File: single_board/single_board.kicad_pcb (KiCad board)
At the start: 4 copper layers, 124.9 x 93.4 mm, 121 parts, among them J1 SWD, J11 SPI Debug, J17 BOOTSEL, J2 USB_C_Receptacle_USB2.0_16P, J30 JST_GH_H, J31 JST_GH_H, J32 PB_Vertical, J33 JST_GH_H, J34 PB_Vertical, J35 JST_GH_H, J36 JST_GH_H, J37 JST_GH_H, J38 PB_Vertical, J39 PB_Vertical, J4 RST, J40 PB_Vertical, J41 PB_Vertical, J42 PB_Vertical, J43 PB_Vertical, J44 PB_Vertical, J45 PB_Vertical, J46 PB_Vertical, J47 PB_Vertical, J48 PB_Vertical, J49 PB_Vertical, J5 JST-GH, J50 PB_Vertical, J6 Conn_01x02, Q1 AO3400A, Q3 AO3401A, SW1 Button, U1 AP2112K-3.3, U3 USBLC6-2SC6, U4 LSM6DSV, U5 STM32G474VBTx, Y2 ABM8-16MHz

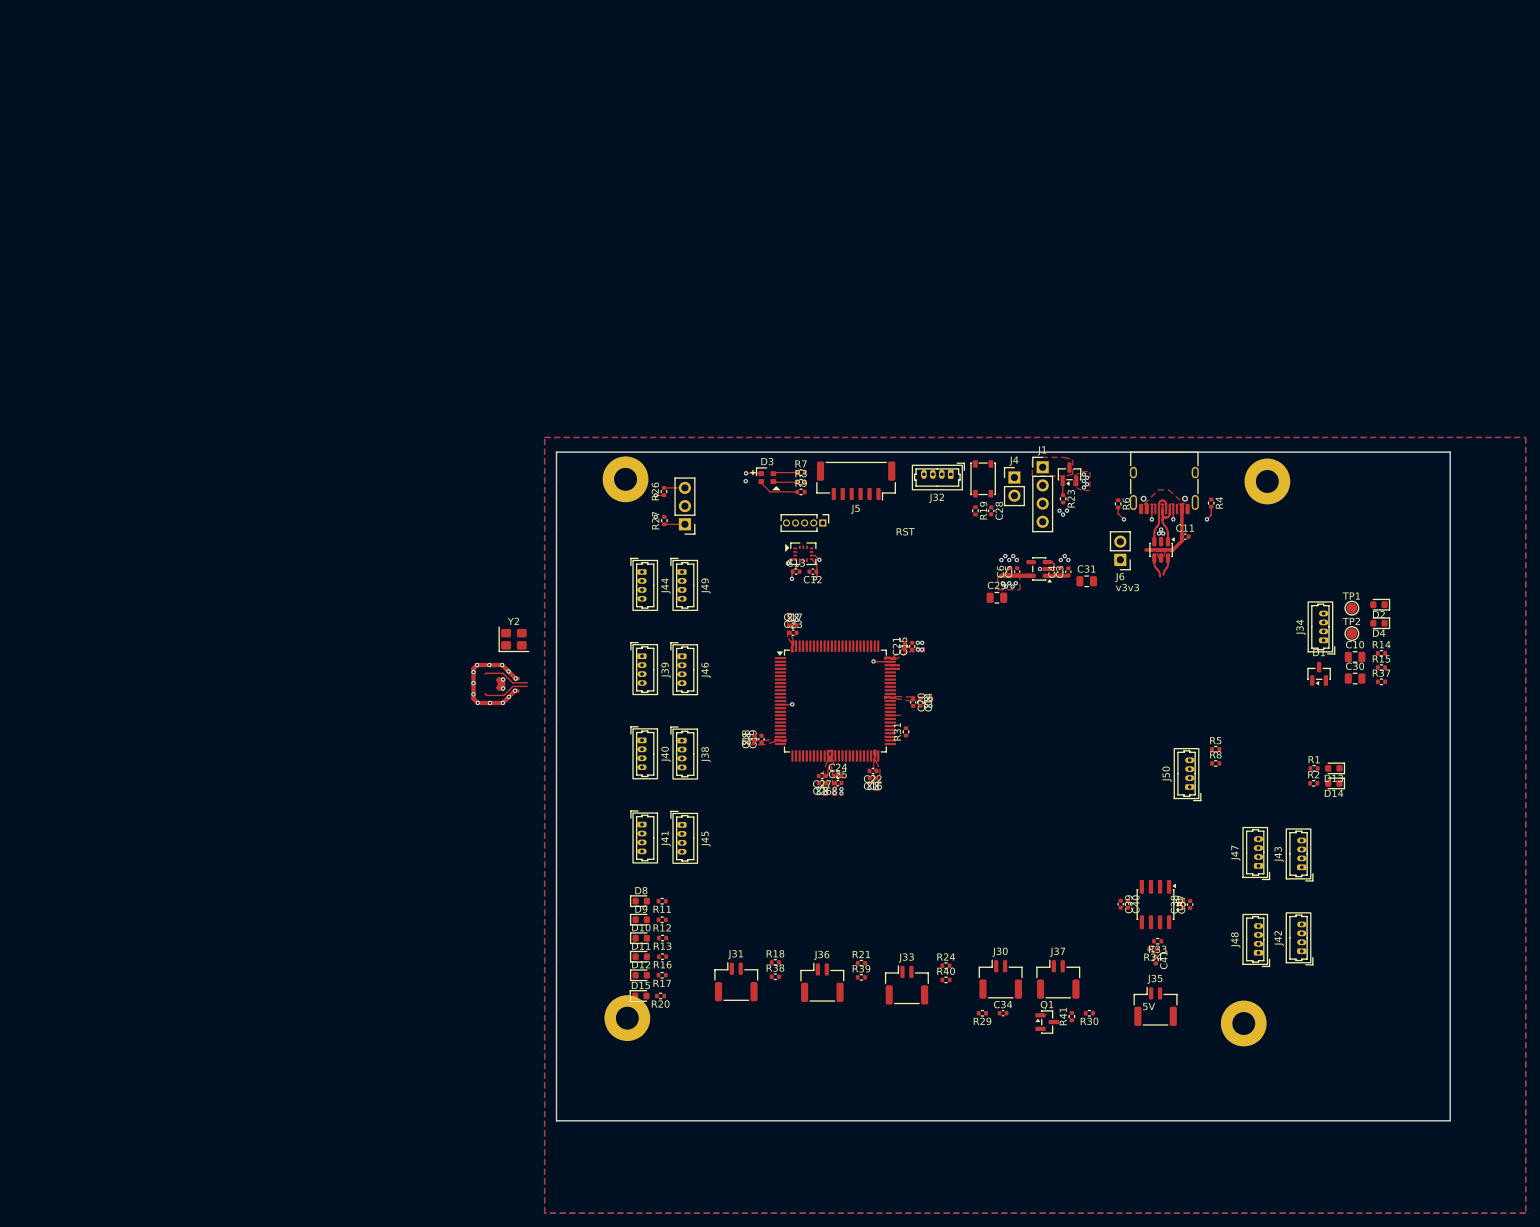
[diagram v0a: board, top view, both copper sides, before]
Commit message: layout positioning
spacing and positioning
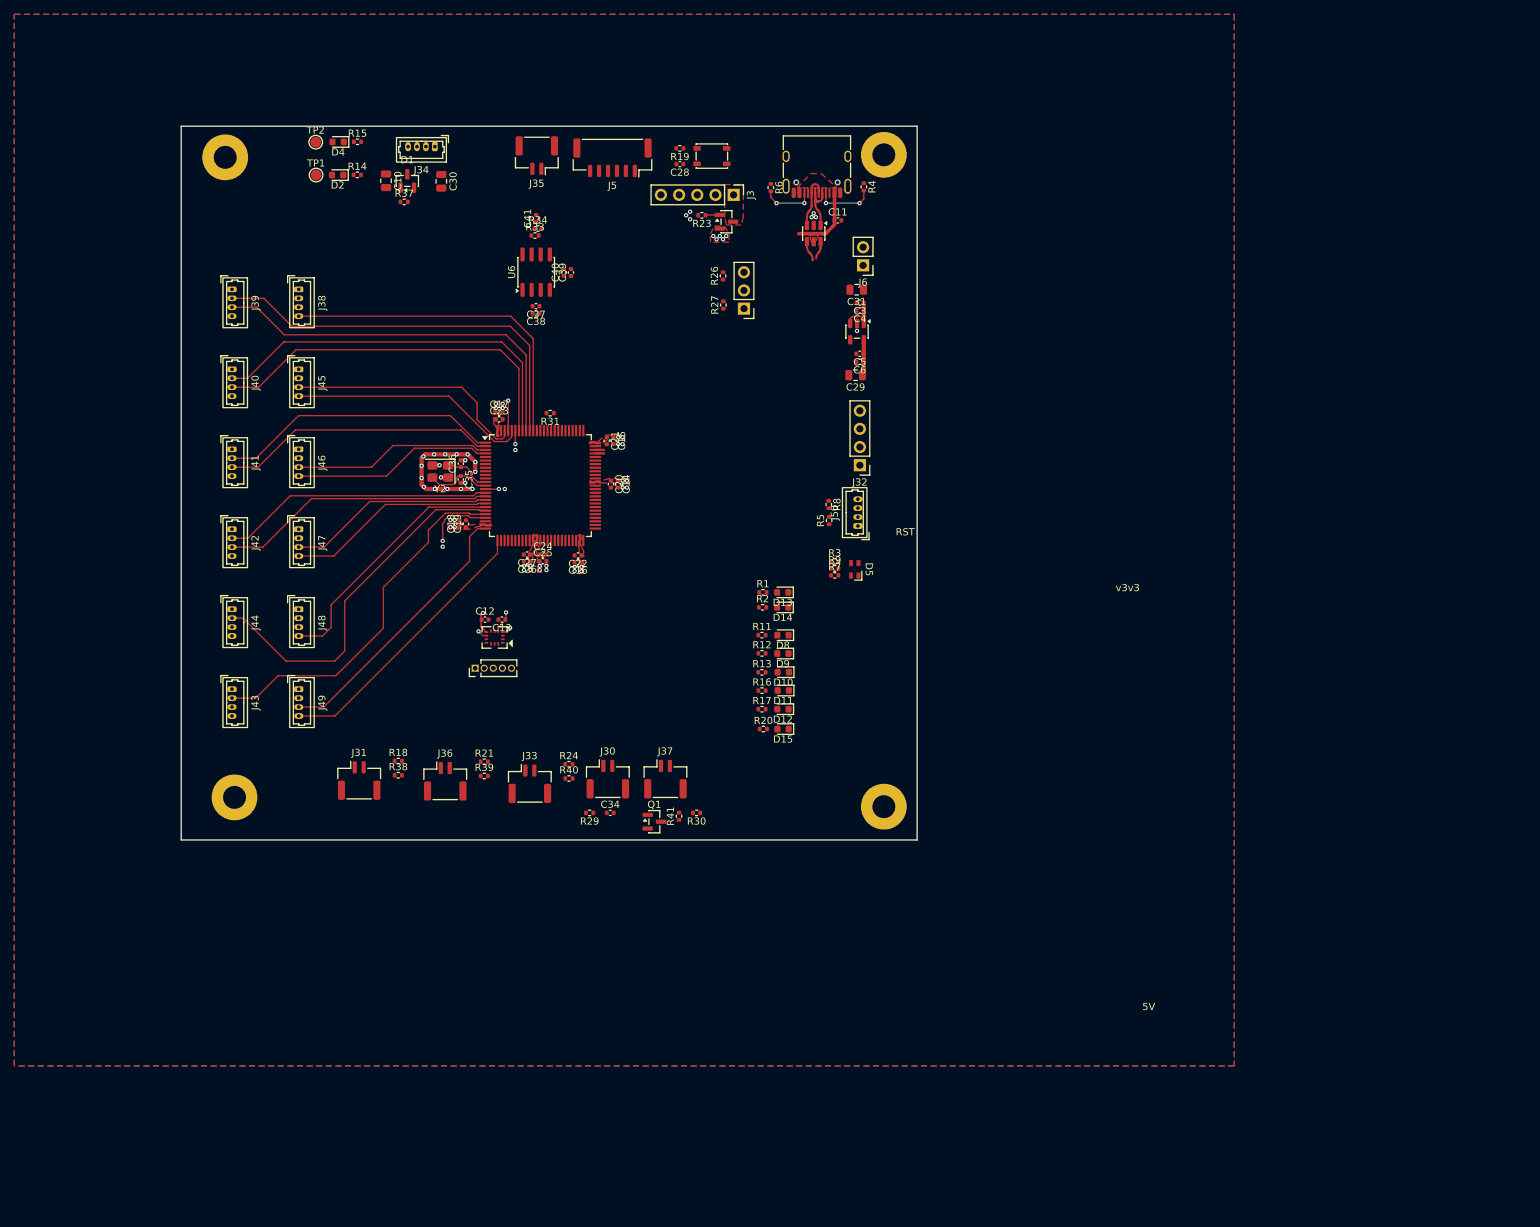
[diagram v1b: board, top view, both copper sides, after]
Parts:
- removed D3: FM-B2020RGBA-HG, rover:FM-B2020RGBA-HG Hand Solder
- removed J1: SWD, Connector_PinHeader_2.54mm:PinHeader_1x04_P2.54mm_Vertical
- removed J4: RST, Connector_PinHeader_2.54mm:PinHeader_1x02_P2.54mm_Vertical
- added C35: 10pF, Capacitor_SMD:C_0402_1005Metric, F.Cu at (97.7, 83.1)
- added C36: 10pF, Capacitor_SMD:C_0402_1005Metric, F.Cu at (97.7, 80.9)
- added D5: TJ-S1615CY6TGLCCSRGB-A5, rover:TOGAILED, F.Cu at (152.7, 95.6)
- added J3: SWD, Connector_PinHeader_2.54mm:PinHeader_1x05_P2.54mm_Vertical, F.Cu at (135.8, 43.3)
- J32: value PB_Vertical -> ~; footprint Connector_Molex:Molex_PicoBlade_53047-0410_1x04_P1.25mm_Vertical -> Connector_PinHeader_2.54mm:PinHeader_1x04_P2.54mm_Vertical
- moved R15 160.9 mm to (83.2, 35.9)
- moved J42 160.7 mm to (65.7, 90.0), turned to -90 degrees
- moved TP2 160.3 mm to (77.4, 35.9)
- moved D4 160.3 mm to (80.5, 35.9)
- moved R14 158.0 mm to (83.2, 40.5)
- moved D2 157.4 mm to (80.5, 40.5)
- moved TP1 156.9 mm to (77.5, 40.5)
- moved R37 152.2 mm to (89.8, 44.3)
- moved J43 151.6 mm to (65.7, 112.4), turned to -90 degrees
- moved C10 150.9 mm to (87.2, 41.3), turned to -90 degrees
- moved J35 147.1 mm to (108.3, 37.8), turned to 180 degrees
- moved C30 145.4 mm to (95.0, 41.4), turned to -90 degrees
- moved D1 144.9 mm to (90.2, 41.4)
- moved J48 142.5 mm to (75.0, 101.2), turned to -90 degrees
- moved J47 142.1 mm to (75.0, 90.0), turned to -90 degrees
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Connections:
- C11 pad 1: /VBUS -> 5V
- C3 pad 1: 5V -> Net-(J6-Pin_1)
- C31 pad 1: 5V -> Net-(J6-Pin_1)
- C4 pad 1: 5V -> Net-(J6-Pin_1)
- D2 pad 1: GND -> Net-(D2-K)
- D2 pad 2: Net-(D2-A) -> 5V
- D4 pad 1: GND -> Net-(D4-K)
- D4 pad 2: Net-(D4-A) -> v3v3
- J2 pad A4: /VBUS -> 5V
- J2 pad A9: /VBUS -> 5V
- J2 pad B4: /VBUS -> 5V
- J2 pad B9: /VBUS -> 5V
- J32 pad 2: /UART4_TX -> /USART1_TX
- J32 pad 3: /UART4_RX -> /USART1_RX
- J39 pad 1: /ENC1_A -> 5V
- J39 pad 2: /ENC1_B -> /ENC1_A
- J39 pad 3: 5V -> /ENC1_B
- J40 pad 1: /ENC2_A -> 5V
- J40 pad 2: /ENC2_B -> /ENC2_A
- J40 pad 3: 5V -> /ENC2_B
- J41 pad 1: /ENC3_A -> 5V
- J41 pad 2: /ENC3_B -> /ENC3_A
- J41 pad 3: 5V -> /ENC3_B
- J42 pad 1: /ENC4_A -> 5V
- J42 pad 2: /ENC4_B -> /ENC4_A
- J42 pad 3: 5V -> /ENC4_B
- J43 pad 1: /ENC5_A -> 5V
- J43 pad 2: /ENC5_B -> /ENC_5
- J43 pad 3: 5V -> GND
- J43 pad 4: GND -> unconnected-(J43-Pin_4-Pad4)
- J44 pad 1: /ENC6_A -> 5V
- J44 pad 2: /ENC6_B -> /ENC_6
- J44 pad 3: 5V -> GND
- J44 pad 4: GND -> unconnected-(J44-Pin_4-Pad4)
- J5 pad 3: /UART5_TX -> /USART3_TX
- J5 pad 4: /UART5_RX -> /USART3_RX
- J6 pad 1: 5V -> Net-(J6-Pin_1)
- J6 pad 2: /VBUS -> 5V
- R14 pad 1: 5V -> Net-(D2-K)
- R14 pad 2: Net-(D2-A) -> GND
- R15 pad 1: v3v3 -> Net-(D4-K)
- R15 pad 2: Net-(D4-A) -> GND
- R3 pad 1: Net-(D3-RK) -> /TRI_LED_B
- R3 pad 2: /TRI_LED_R -> Net-(D5-BA)
- R7 pad 1: Net-(D3-GK) -> /TRI_LED_G
- R7 pad 2: /TRI_LED_G -> Net-(D5-GA)
- R9 pad 1: Net-(D3-BK) -> /TRI_LED_R
- R9 pad 2: /TRI_LED_B -> Net-(D5-RA)
- U1 pad 1: 5V -> Net-(J6-Pin_1)
- U1 pad 3: 5V -> Net-(J6-Pin_1)
- U3 pad 5: /VBUS -> 5V
- U5 pad 1: /ENC6_A -> /ENC3_A
- U5 pad 15: /ENC1_A -> /ENC4_A
- U5 pad 16: /ENC1_B -> /ENC4_B
- U5 pad 17: /PWM1 -> /PWM4
- U5 pad 18: /DIR1 -> /DIR4
- U5 pad 19: unconnected-(U5-PF2-Pad19) -> /DIR5
- U5 pad 2: /ENC6_B -> /ENC3_B
- U5 pad 20: /ENC2_A -> /ENC_6
- U5 pad 21: /ENC2_B -> /ENC_5
- U5 pad 22: unconnected-(U5-PA2-Pad22) -> /PWM5
- U5 pad 25: /PWM2 -> /PWM6
- U5 pad 26: /DIR2 -> /DIR6
- U5 pad 27: /LED1 -> /IMU_SCK
- U5 pad 28: /ENC3_A -> /IMU_MISO
- U5 pad 29: /ENC3_B -> /IMU_MOSI
- U5 pad 3: unconnected-(U5-PE4-Pad3) -> /PWM3
- U5 pad 30: /LED2 -> /IMU_NSS
- U5 pad 31: /LED3 -> /INT1
- U5 pad 32: /LED4 -> /INT2
- U5 pad 33: /LED5 -> unconnected-(U5-PB1-Pad33)
- U5 pad 34: /LED6 -> unconnected-(U5-PB2-Pad34)
- U5 pad 4: /PWM3 -> /DIR3
- U5 pad 42: unconnected-(U5-PE11-Pad42) -> /LASER_SIG
- U5 pad 46: /LASER_SIG -> unconnected-(U5-PE15-Pad46)
- U5 pad 5: /DIR3 -> unconnected-(U5-PE6-Pad5)
- U5 pad 51: /CAN_RX -> /LED6
- U5 pad 52: /CAN_TX -> /LED5
- U5 pad 53: /CAN_STB -> /LED4
- U5 pad 54: /CAN_LED -> /LED3
- U5 pad 55: /HEARTBEAT -> /LED2
- U5 pad 56: unconnected-(U5-PD9-Pad56) -> /LED1
- U5 pad 57: unconnected-(U5-PD10-Pad57) -> /HEARTBEAT
- U5 pad 58: unconnected-(U5-PD11-Pad58) -> /CAN_LED
- U5 pad 59: /ENC4_A -> unconnected-(U5-PD12-Pad59)
- U5 pad 60: /ENC4_B -> unconnected-(U5-PD13-Pad60)
- U5 pad 61: /DIR5 -> unconnected-(U5-PD14-Pad61)
- U5 pad 62: /PWM5 -> unconnected-(U5-PD15-Pad62)
- U5 pad 65: /ENC5_A -> /TRI_LED_G
- U5 pad 66: /ENC5_B -> /TRI_LED_R
- U5 pad 67: /PWM4 -> /TRI_LED_B
- U5 pad 68: /DIR4 -> /I2C_SDA
- U5 pad 69: /I2C_SDA -> /I2C_SCL
- U5 pad 70: /I2C_SCL -> /USART1_TX
- U5 pad 71: unconnected-(U5-PA10-Pad71) -> /USART1_RX
- U5 pad 79: /UART4_TX -> /USART3_TX
- U5 pad 80: /UART4_RX -> /USART3_RX
- U5 pad 81: /UART5_TX -> unconnected-(U5-PC12-Pad81)
- U5 pad 82: unconnected-(U5-PD0-Pad82) -> /CAN_RX
- U5 pad 83: unconnected-(U5-PD1-Pad83) -> /CAN_TX
- U5 pad 84: /UART5_RX -> /CAN_STB
- U5 pad 85: /TRI_LED_G -> unconnected-(U5-PD3-Pad85)
- U5 pad 86: /TRI_LED_R -> unconnected-(U5-PD4-Pad86)
- U5 pad 87: /TRI_LED_B -> unconnected-(U5-PD5-Pad87)
- U5 pad 88: /INT2 -> unconnected-(U5-PD6-Pad88)
- U5 pad 89: /IMU_NSS -> unconnected-(U5-PD7-Pad89)
- U5 pad 90: /IMU_SCK -> /DIR1
- U5 pad 91: /IMU_MISO -> /ENC1_A
- U5 pad 92: /IMU_MOSI -> /ENC1_B
- U5 pad 93: /INT1 -> /ENC2_A
- U5 pad 94: unconnected-(U5-PB7-Pad94) -> /ENC2_B
- U5 pad 96: unconnected-(U5-PB9-Pad96) -> /DIR2
- U5 pad 97: /DIR6 -> /PWM1
- U5 pad 98: /PWM6 -> /PWM2
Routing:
- net /ENC1_A: track 0.00 -> 56.2 mm
- net /ENC1_B: track 0.00 -> 54.5 mm
- net /ENC2_A: track 0.00 -> 53.4 mm
- net /ENC2_B: track 0.00 -> 52.0 mm
- net /ENC_6: track 0.00 -> 50.8 mm
- net /ENC_5: track 0.00 -> 50.5 mm
- net /DIR1: track 0.00 -> 46.9 mm
- net /ENC3_A: track 0.00 -> 39.5 mm
- net /DIR6: track 0.00 -> 39.0 mm
- net /ENC3_B: track 0.00 -> 38.5 mm
- net /PWM6: track 0.00 -> 38.5 mm
- net /ENC4_B: track 0.00 -> 38.4 mm
- net /ENC4_A: track 1.40 -> 38.1 mm
- net /DIR5: track 0.00 -> 35.4 mm
- net /PWM2: track 0.00 -> 34.1 mm
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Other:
- board size 124.9 x 93.4 mm -> 102.8 x 99.7 mm
